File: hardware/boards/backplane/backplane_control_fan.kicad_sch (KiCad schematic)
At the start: 41 parts, among them J13 FAN_3PIN, Q1 Q_PMOS_GSD, Q2 Q_NPN_BEC, U1 TCA9548APWR, U2 WT32-ETH01

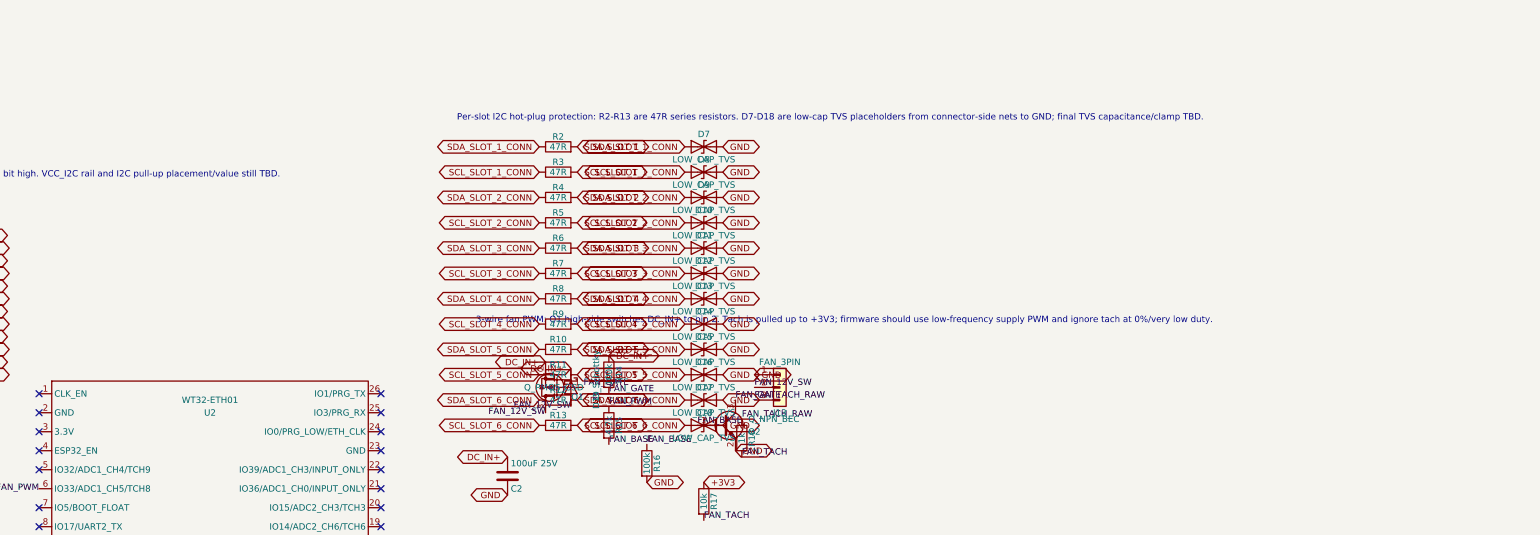
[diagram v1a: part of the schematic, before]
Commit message: Starrting to move things around
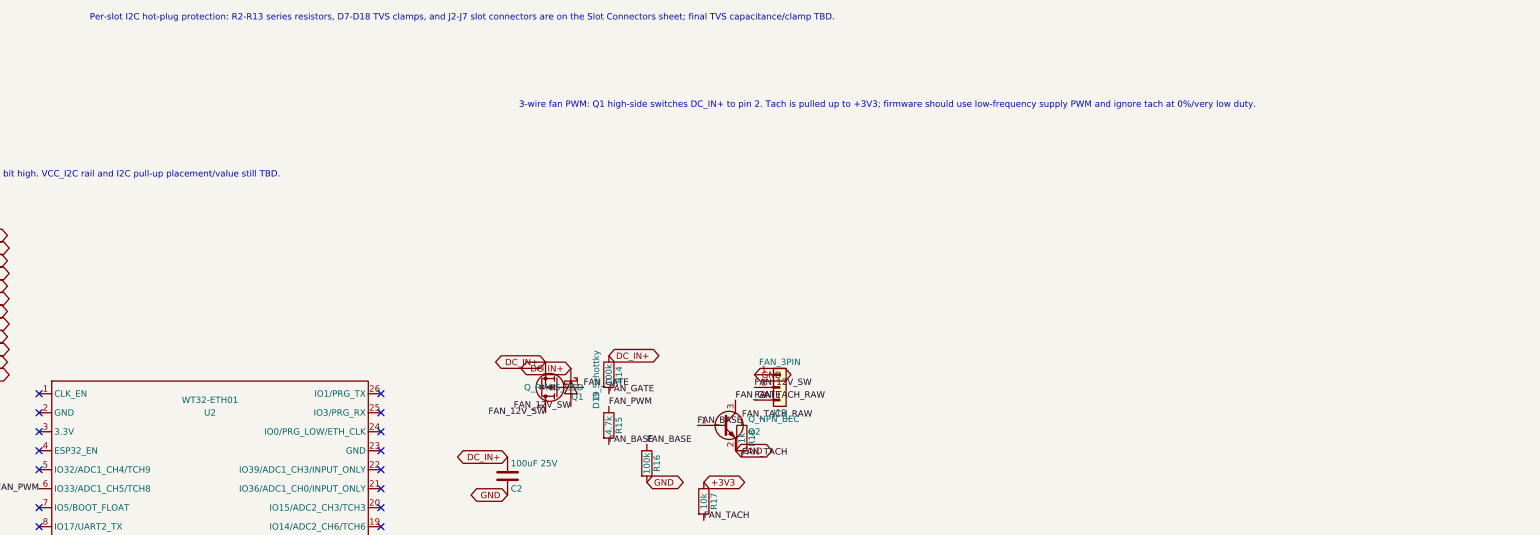
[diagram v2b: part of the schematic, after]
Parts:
- removed D10, D11, D12, D13, D14, D15, D16, D17, D18, D7, D8, D9: LOW_CAP_TVS, Diode_SMD:D_SOD-523, symbol Device:D_TVS
- removed R10, R11, R12, R13, R2, R3, R4, R5, R6, R7, R8, R9: 47R, Resistor_SMD:R_0603_1608Metric, symbol Device:R
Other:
- note added: "Per-slot I2C hot-plug protection: R2-R13 series resistors, D7-D18 TVS clamps, and J2-J7 slot connectors are on the Slot Connectors sheet; final TVS capacitance/clamp TBD."
- note removed: "Per-slot I2C hot-plug protection: R2-R13 are 47R series resistors. D7-D18 are low-cap TVS placeholders from connector-side nets to GND; final TVS capacitance/clamp TBD."

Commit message: Clean up the backplane schematic
And start over with the PCB using a bit saner layout
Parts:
- removed C2: 100uF 25V, Capacitor_THT:CP_Radial_D6.3mm_P2.50mm, symbol Device:C
- removed U2: WT32-ETH01, WT32-ETH01:WT32-ETH01, symbol WT32-ETH01:WT32-ETH01
- added J1: SPARE_I2C, symbol Connector_Generic:Conn_01x04
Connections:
- net at U1.17 (SD6): now also J1.2 (Pin_2)
- net at U1.18 (SC6): now also J1.1 (Pin_1)
- net at U1.19 (SD7): now also J1.4 (Pin_4)
- net at U1.20 (SC7): now also J1.3 (Pin_3)
- net DC_IN+ renamed +12V
- net FAN_BASE: no longer names the net of Q2.1 (B), R15.2, R16.1
- net FAN_GATE: no longer names the net of Q1.1 (G), Q2.3 (C), R14.2
- net FAN_TACH_RAW: no longer names the net of J13.3 (Pin_3), R18.1
- no-connect marks 28 -> 0
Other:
- note added: "SCL/SDA for port 6 and 7 for future expansion use"
- note added: "TCA9548A: JP1-JP3 default A0/A1/A2 low for 0x70; cut 1-2 and bridge 1-3 to set a bit high."
- note added: "TODO: schottky needed if it's built in to the FET?"
- note removed: "Per-slot I2C hot-plug protection: R2-R13 series resistors, D7-D18 TVS clamps, and J2-J7 slot connectors are on the Slot Connectors sheet; final TVS capacitance/clamp TBD."
- note removed: "TCA9548A: JP1-JP3 default A0/A1/A2 low for 0x70; cut 1-2 and bridge 1-3 to set a bit high. VCC_I2C rail and I2C pull-up placement/value still TBD."
- moved on the sheet: C1, J13, Q1, Q2, R1, R15, R17, R18, U1
